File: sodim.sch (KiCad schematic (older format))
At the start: 1 part, among them J1 ddr4-sodimm-edge-connector

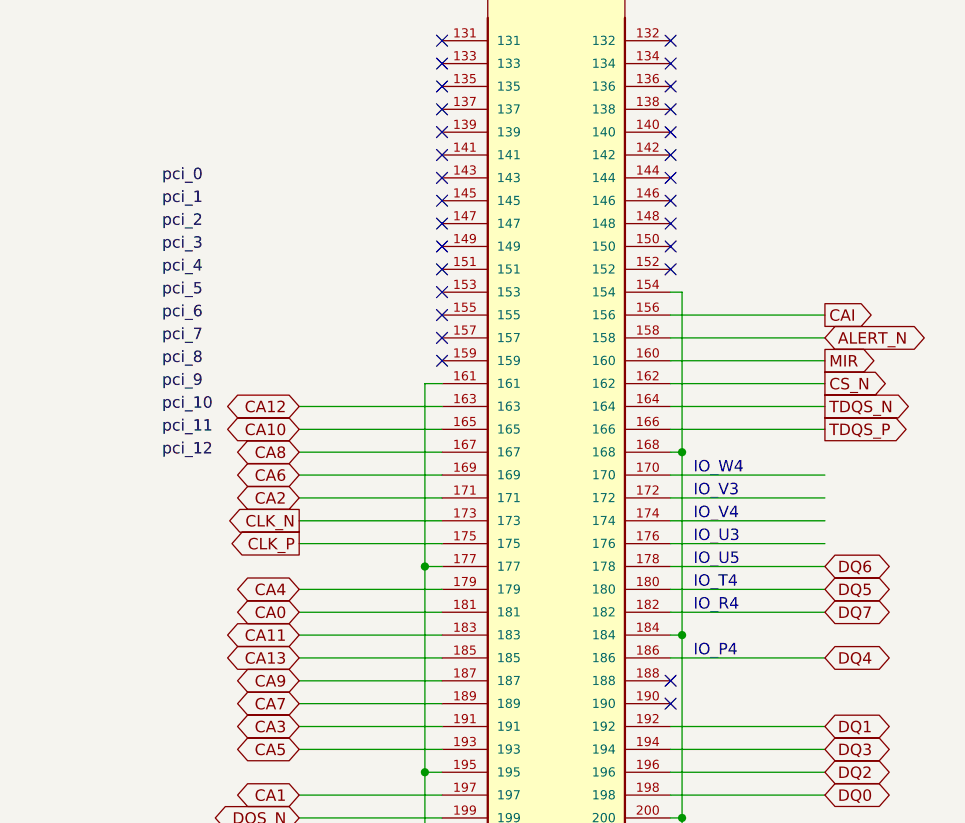
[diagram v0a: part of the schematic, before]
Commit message: Cleanup
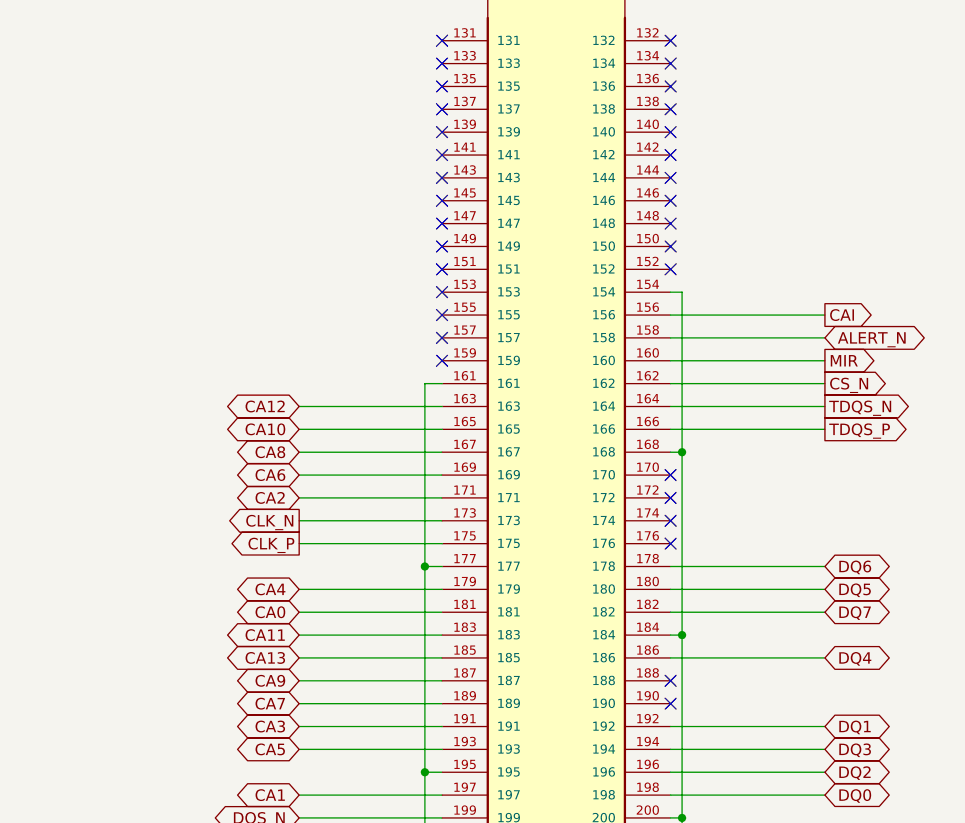
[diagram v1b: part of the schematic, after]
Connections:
- no-connect marks 144 -> 148
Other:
- note removed: "IO_P4"
- note removed: "IO_R4"
- note removed: "IO_T4"
- note removed: "IO_U3"
- note removed: "IO_U5"
- note removed: "IO_V3"
- note removed: "IO_V4"
- note removed: "IO_W4"
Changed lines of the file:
@@
 	1    0    0    -1
 $EndComp
-Text Notes 10600 5300 0    50   ~ 0
-IO_P4
-Text Notes 10600 5100 0    50   ~ 0
-IO_R4
-Text Notes 10600 5000 0    50   ~ 0
-IO_T4
-Text Notes 10600 4900 0    50   ~ 0
-IO_U5
-Text Notes 10600 4800 0    50   ~ 0
-IO_U3
-Text Notes 10600 4700 0    50   ~ 0
-IO_V4
-Text Notes 10600 4600 0    50   ~ 0
-IO_V3
-Text Notes 10600 4500 0    50   ~ 0
-IO_W4
 Wire Wire Line
 	10500 5300 11175 5300
@@
 Wire Wire Line
 	10500 4100 11175 4100
-Wire Wire Line
-	10500 4700 11175 4700
-Wire Wire Line
-	10500 4800 11175 4800
-Wire Wire Line
-	10500 4500 11175 4500
-Wire Wire Line
-	10500 4600 11175 4600
 $Comp
 L ddr5-testbed:ddr4-sodimm-edge-connector J1
@@
 Wire Wire Line
 	10500 6300 11175 6300
-Text Label 8275 3225 0    50   ~ 0
-pci_0
-Text Label 8275 3325 0    50   ~ 0
-pci_1
-Text Label 8275 3425 0    50   ~ 0
-pci_2
-Text Label 8275 3525 0    50   ~ 0
-pci_3
-Text Label 8275 3625 0    50   ~ 0
-pci_4
-Text Label 8275 3725 0    50   ~ 0
-pci_5
-Text Label 8275 3825 0    50   ~ 0
-pci_6
-Text Label 8275 3925 0    50   ~ 0
-pci_7
-Text Label 8275 4025 0    50   ~ 0
-pci_8
-Text Label 8275 4125 0    50   ~ 0
-pci_9
-Text Label 8275 4225 0    50   ~ 0
-pci_10
-Text Label 8275 4325 0    50   ~ 0
-pci_11
-Text Label 8275 4425 0    50   ~ 0
-pci_12
+NoConn ~ 10500 4500
+NoConn ~ 10500 4600
+NoConn ~ 10500 4700
+NoConn ~ 10500 4800
 $EndSCHEMATC
